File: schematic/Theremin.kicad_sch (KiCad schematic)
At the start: 56 parts, among them Q1 2N7002, Q10 BC817, Q2 2N7002, Q3 2N7002, Q4 BC817, Q5 BC817, Q6 2N7002, Q7 2N7002, Q8 2N7002, Q9 BC817, U1 NE555D, U2 AZV3002, U3 MAX4392, U4 MAX4392, U5 NE555D, U6 AZV3002

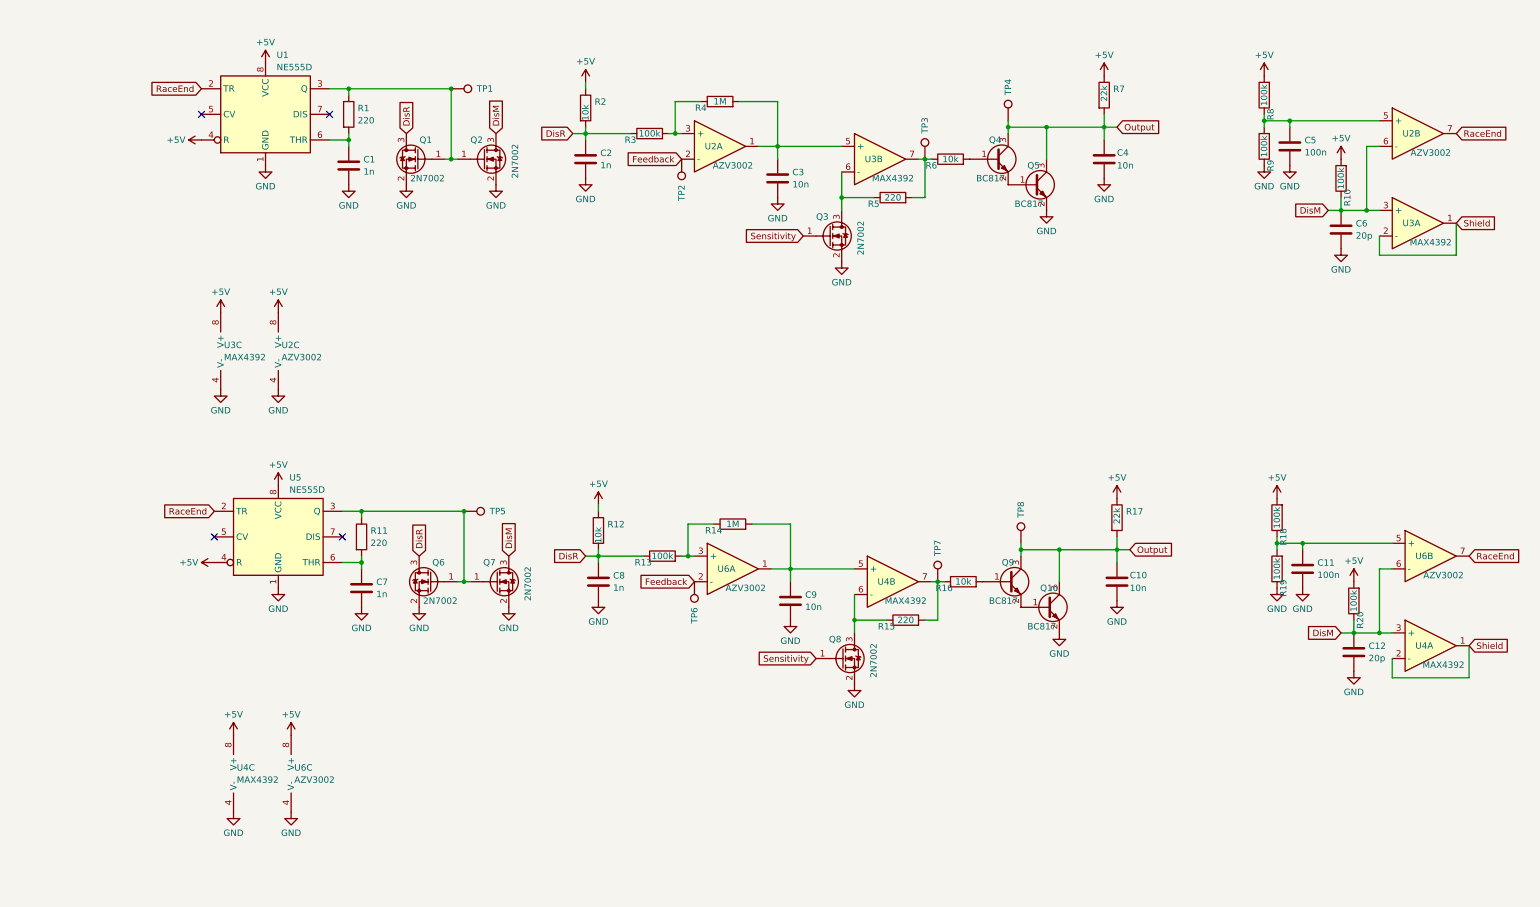
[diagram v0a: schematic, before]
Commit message: Continued schematic
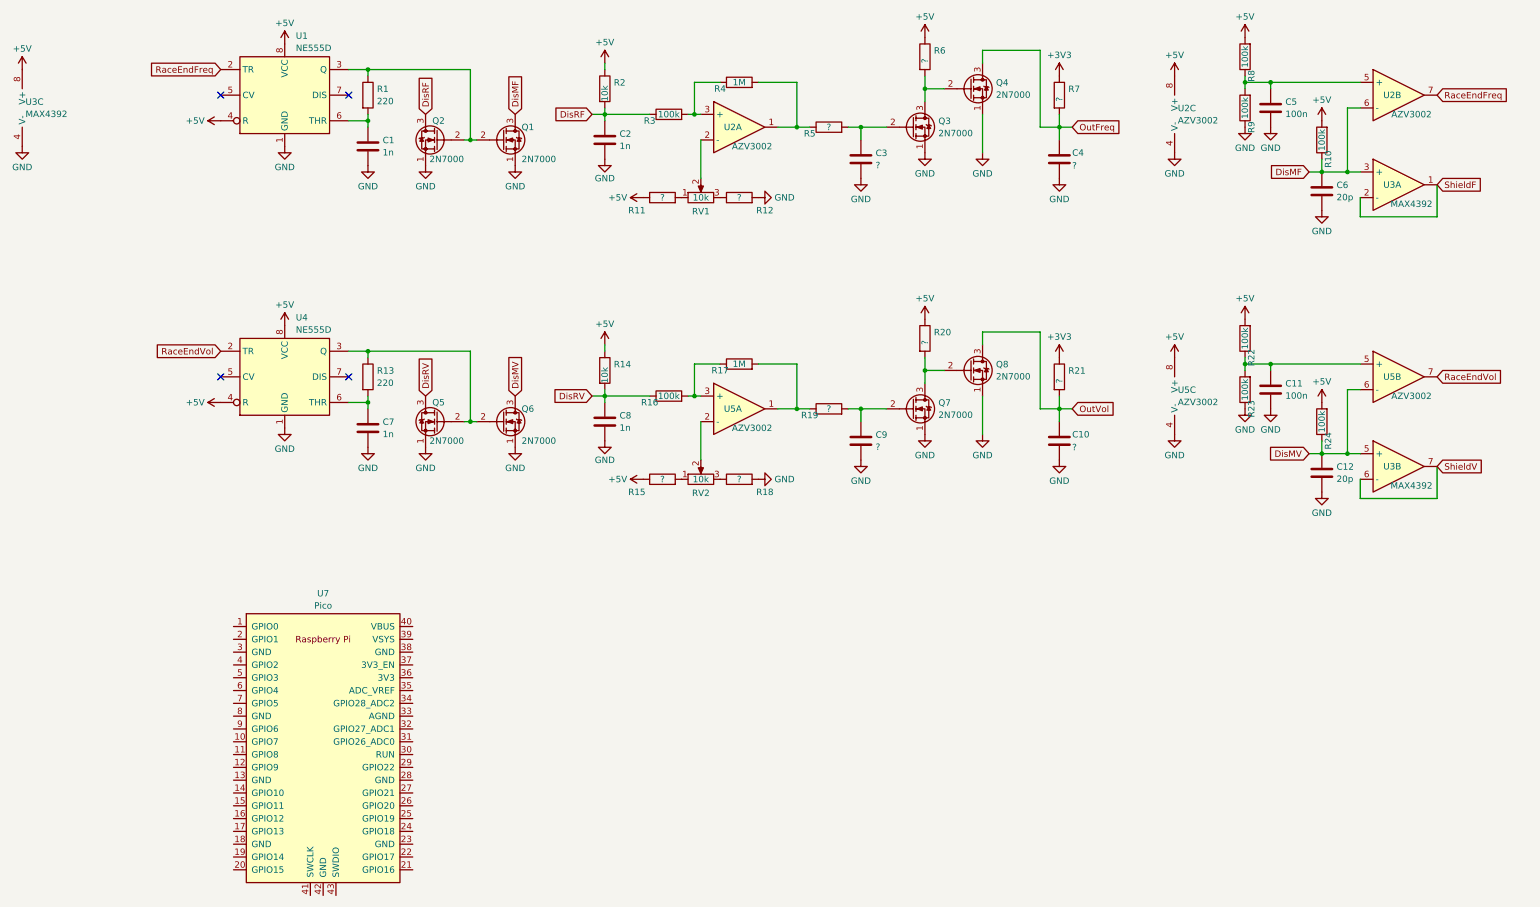
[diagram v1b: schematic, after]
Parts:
- removed Q1, Q2, Q3, Q6, Q7, Q8: 2N7002, Package_TO_SOT_SMD:SOT-23, symbol Transistor_FET:2N7002
- removed Q10, Q4, Q5, Q9: BC817, Package_TO_SOT_SMD:SOT-23, symbol Transistor_BJT:BC817
- removed TP1, TP2, TP3, TP4, TP5, TP6, TP7, TP8: TestPoint, TestPoint:TestPoint_Pad_D1.5mm, symbol Connector:TestPoint
- removed U4: MAX4392, Package_SO:SOIC-8_3.9x4.9mm_P1.27mm, symbol Device:Opamp_Dual
- removed U5: NE555D, Package_SO:SOIC-8_3.9x4.9mm_P1.27mm, symbol Timer:NE555D
- removed U6: AZV3002, Package_SO:SOIC-8_3.9x4.9mm_P1.27mm, symbol Device:Opamp_Dual
- added Q1, Q2, Q3, Q4, Q5, Q6, Q7, Q8: 2N7000, Package_TO_SOT_THT:TO-92_Inline, symbol Transistor_FET:2N7000
- added R21: ?, Resistor_SMD:R_0805_2012Metric, symbol Device:R
- added R22, R23, R24: 100k, Resistor_SMD:R_0805_2012Metric, symbol Device:R
- added RV1, RV2: 10k, symbol Device:R_Potentiometer
- added U4: NE555D, Package_SO:SOIC-8_3.9x4.9mm_P1.27mm, symbol Timer:NE555D
- added U5: AZV3002, Package_SO:SOIC-8_3.9x4.9mm_P1.27mm, symbol Device:Opamp_Dual
- added U7: Pico, RPi_Pico:RPi_Pico_SMD_TH, symbol Pico:Pico
- C10, C3, C4, C9: value 10n -> ?
- R11, R15, R5: value 220 -> ?
- R12, R6: value 10k -> ?
- R13: value 100k -> 220
- R14: value 1M -> 10k
- R16: value 10k -> 100k
- R17: value 22k -> 1M
- R18, R19, R20: value 100k -> ?
- R7: value 22k -> ?
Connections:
- net +5V: now also R11.1, R14.1, R15.1, R20.1, R6.1, R22.2, R24.2, U4.4 (R), U4.8 (VCC), U5.8 (V+); no longer R12.1, R17.1, R18.2, R20.2, R7.1
- net GND: now also R12.2, R18.2, Q1.1 (S), Q2.1 (S), Q3.1 (S), Q4.1 (S), Q5.1 (S), Q6.1 (S), Q7.1 (S), Q8.1 (S), R23.1, U4.1 (GND), U5.4 (V-); no longer R19.1
- net at C9.1: now also R19.2, Q7.2 (G); no longer R14.2
- net at R13.2: now also C7.1, U4.6 (THR); no longer R14.1
- net at R1.1, U1.3 (Q): now also Q1.2 (G), Q2.2 (G)
- net at R11.2: now also RV1.1; no longer C7.1
- net at R15.2: now also RV2.1; no longer R16.1
- net at R16.2: now also R17.1, U5.3 (+)
- net at R4.2, U2.1: now also R5.1; no longer C3.1, U3.5 (+)
- net ShieldV: now reaches U3.6 (-)
- net ShieldV: now also U3.7; no longer R5.1
- net at R6.2: now also Q3.3 (D), Q4.2 (G)
- net DisM renamed DisMF
- net DisMF: now also Q1.3 (D); no longer C12.1, R20.1
- net DisR renamed DisRF
- net DisRF: now also Q2.3 (D); no longer C8.1, R12.2, R13.1
- net Feedback: no longer names the net of U2.2 (-)
- net Feedback: now also RV1.2
- net Output renamed OutFreq
- net OutFreq: now also Q4.3 (D); no longer C10.1, R17.2
- net RaceEnd renamed RaceEndFreq
- net Shield renamed ShieldF
- new net: R17.2, R19.1, U5.1
- new net: RV2.2, U5.2 (-)
- new net: Q5.2 (G), Q6.2 (G), R13.1, U4.3 (Q)
- new net: R12.1, RV1.3
- new net: C3.1, Q3.2 (G), R5.2
- new net: C11.1, R22.1, R23.2, U5.5 (+)
- new net: R18.1, RV2.3
- new net: Q7.3 (D), Q8.2 (G), R20.2
- new net +3V3: R21.1, R7.1
- new net DisMV: C12.1, Q6.3 (D), R24.1, U3.5 (+), U5.6 (-)
- new net DisRV: C8.1, Q5.3 (D), R14.2, R16.1
- new net OutVol: C10.1, Q8.3 (D), R21.2
- new net RaceEndVol: U4.2 (TR), U5.7
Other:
- moved on the sheet: C1, C2, C3, C4, C5, C6, R1, R10, R2, R3, R4, R7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
